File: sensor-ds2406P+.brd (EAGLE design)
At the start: 31.1 x 19.1 mm, 14 parts, among them IC1 DS2406P+

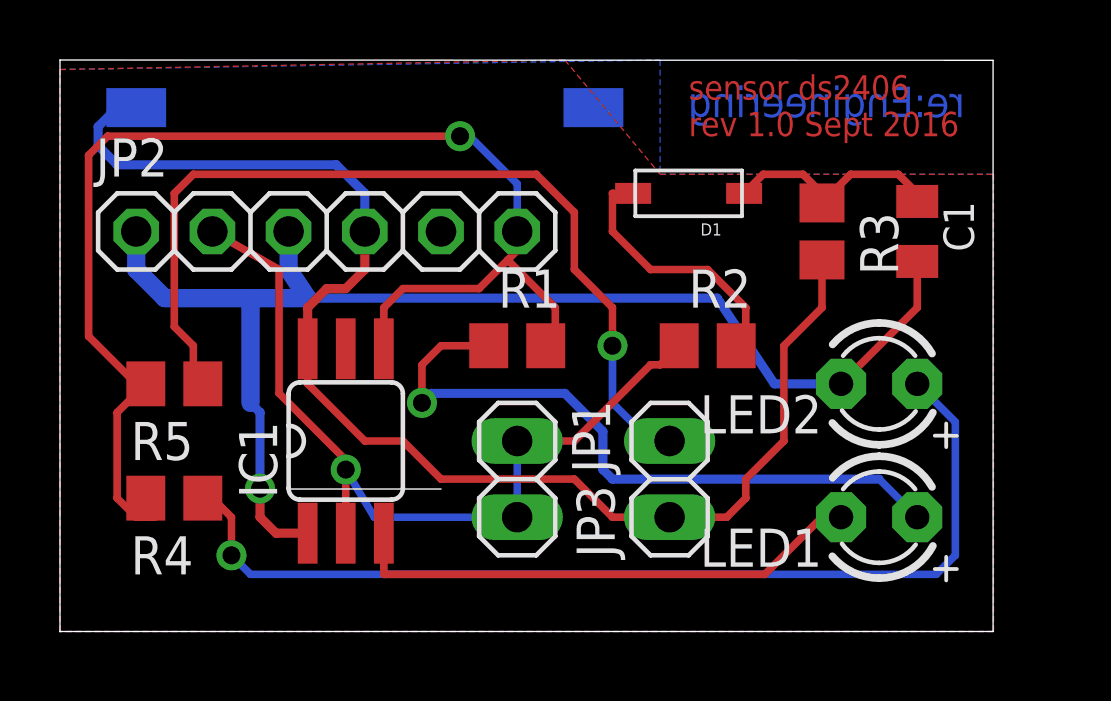
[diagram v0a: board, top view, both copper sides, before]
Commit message: Add files via upload
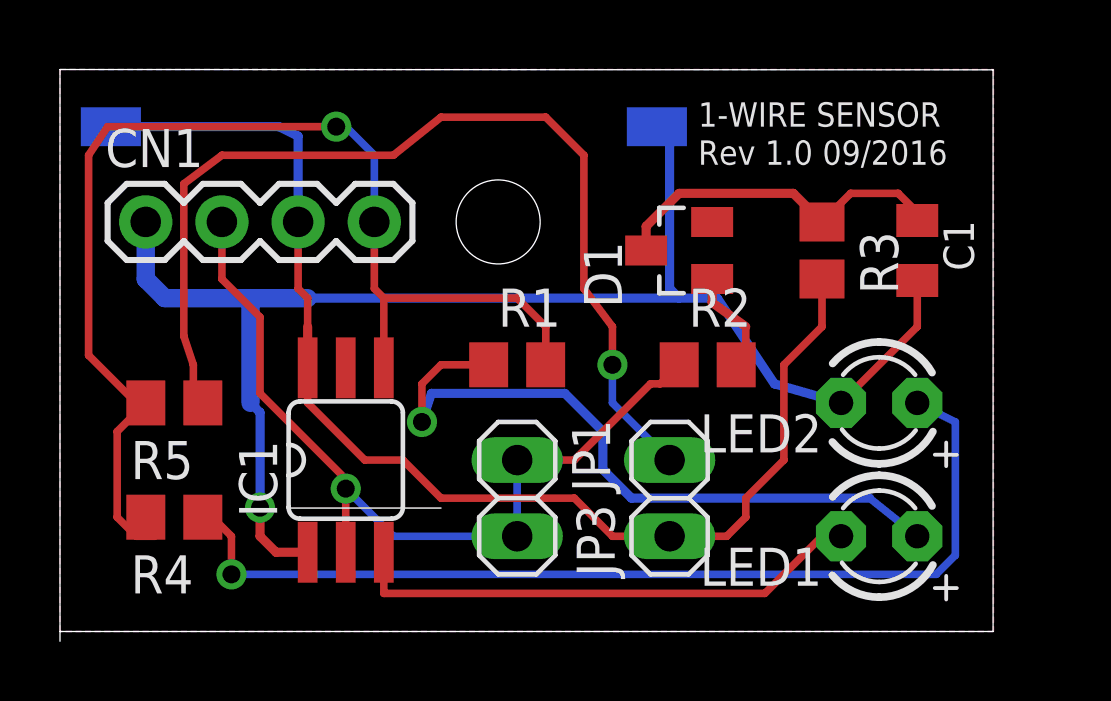
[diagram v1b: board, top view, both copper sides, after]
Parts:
- removed JP2: IF, adafruit:1X06
- removed S1: REED-SWITCH-CT10-1530-G1, switch-reed:CT10-G1
- added CN1: (no value), adafruit:1X04-BIG
- added S5: REED-SWITCH, switch-reed:MK15
- D1: value xx -> 1N4148; device adafruit:SOD-123 -> dont:SOT23
- moved D1 1.93 mm to (20.6, 12.7), turned to 90 degrees
- moved C1 0.64 mm to (28.6, 12.7)
- moved R3 0.64 mm to (25.4, 12.7)
- moved LED2 0.64 mm to (27.3, 7.62)
- moved R5 0.64 mm to (3.81, 7.62)
- moved LED1 0.64 mm to (27.3, 3.17)
- moved R4 0.64 mm to (3.81, 3.81)
- moved IC1 0.63 mm to (10.2, 5.71)
- moved JP1 0.63 mm to (15.2, 4.45)
- moved JP3 0.63 mm to (20.3, 4.45)
- moved R1 0.63 mm to (15.2, 8.89)
- moved R2 0.63 mm to (21.6, 8.89)
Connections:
- net GND: now also CN1.1, S5.2; no longer JP2.1, JP2.3, S1.2
- net IO: now also CN1.2; no longer JP2.2
- net N$2: now also D1.1; no longer D1.A
- net N$5: now also D1.3; no longer D1.C
- net PIO$B: now also CN1.3, S5.1; no longer JP2.4, S1.1
- net VDD: now also CN1.4; no longer JP2.6
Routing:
- net GND: track 43.5 -> 53.3 mm
- net N$2: track 8.86 -> 3.57 mm
- net N$5: track 7.54 -> 11.6 mm
- net PIO$B: track 45.7 -> 41.8 mm
- net N$7: track 30.2 -> 33.4 mm
- net VDD: track 42.0 -> 39.7 mm
- net N$1: track 22.9 -> 23.6 mm
- net N$6: track 33.4 -> 32.7 mm
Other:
- outline, holes or cut-outs redrawn
- board text added: "1-WIRE SENSOR"
- board text added: "Rev 1.0 09/2016"
- board text added: "S5"
- board text removed: "sensor ds2406 rev 1.0 Sept 2016"
